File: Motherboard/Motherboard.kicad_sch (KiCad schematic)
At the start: 57 parts, among them J1 40-pin IDE Connector, J3 Bus_ISA_8bit, J4 ATX-24, J5 USB_B, J6 ATF15XX_JTAG_ISP, J7 Bus_ISA_8bit, J8 65SIB_Connector, SW1 SW_Push, SW2 SW_SPST, U1 AS6C8008, U10 ATF1508AS-PLCC84, U11 74HCT245, U12 74HCT573, U13 8255, U14 WD65C22, U15 AS6C8008, U16 MCP2200-I-SO, U17 74HCT163, U18 LM7905_TO220, U19 GAL16V8, U2 74HCT04, U4 SST39SF040, U5 SST39SF040, U6 SST39SF040, U7 SST39SF040, U8 WD65C816S, U9 DS1813, X1 ACO-xxxMHz, X2 ACO-24MHz, X3 ACO-14.31818MHz

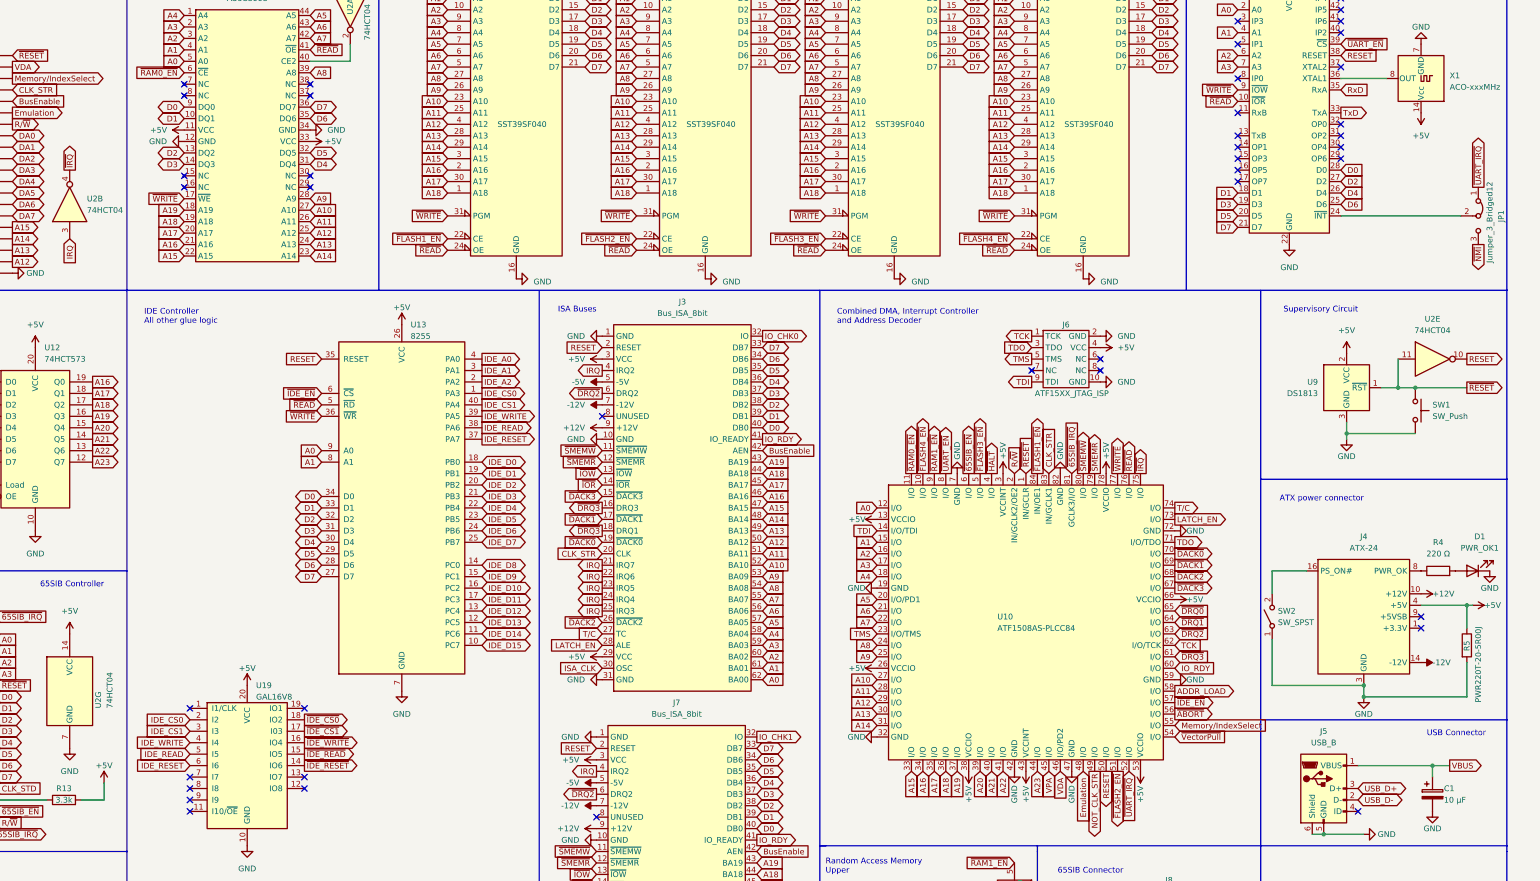
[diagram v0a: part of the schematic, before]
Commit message: Updated component footprints...
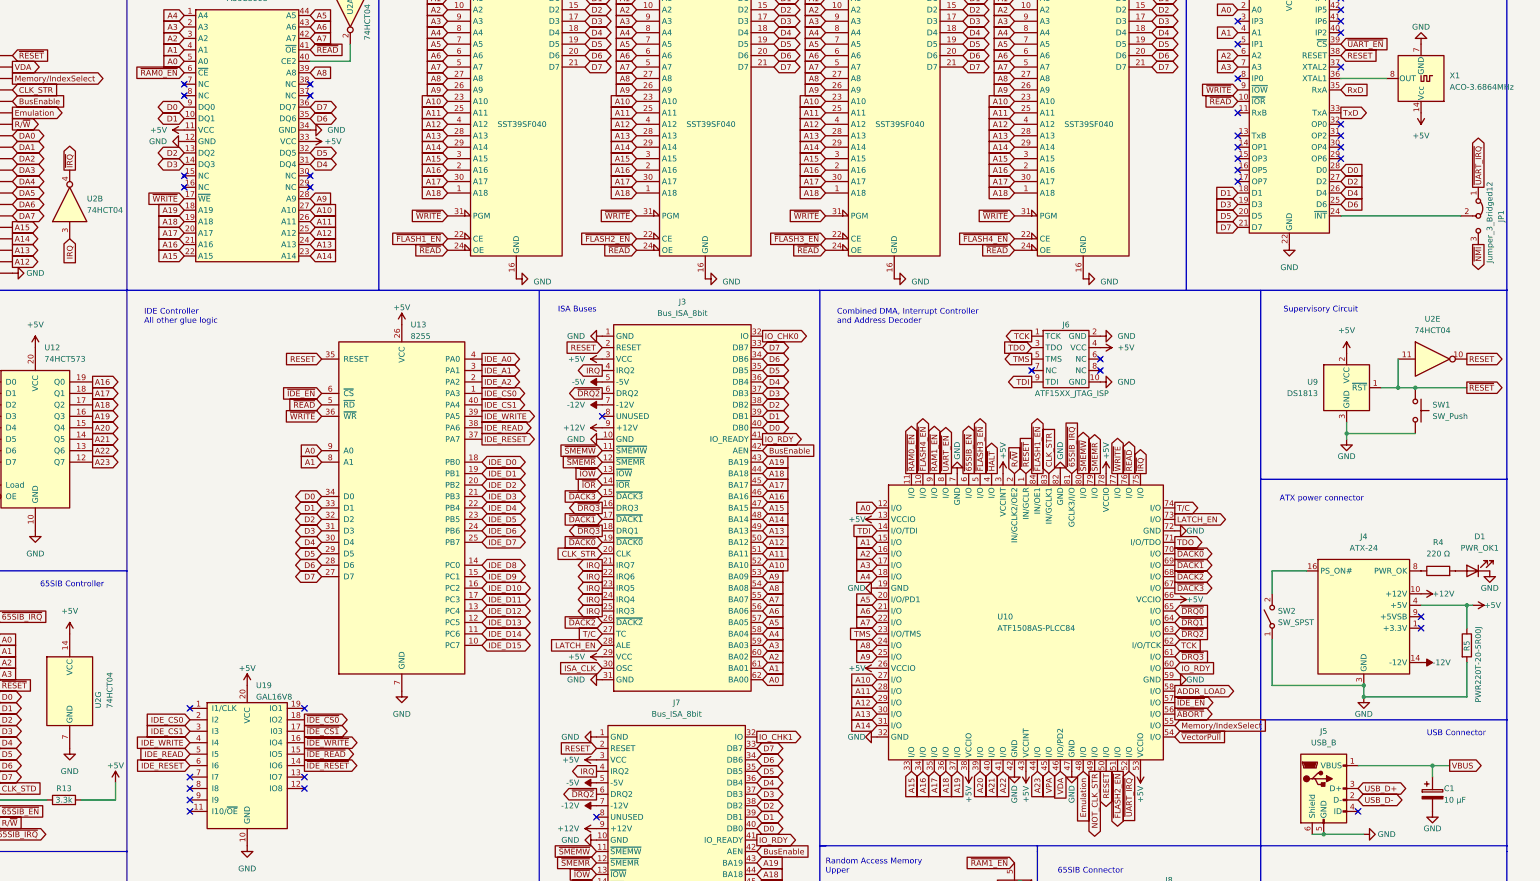
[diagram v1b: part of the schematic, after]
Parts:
- D7: footprint (none) -> LED_THT:LED_D5.0mm
- R12: footprint (none) -> Resistor_THT:R_Axial_DIN0207_L6.3mm_D2.5mm_P7.62mm_Horizontal
- U3: footprint (none) -> Package_LCC:PLCC-44_THT-Socket
- X1: value ACO-xxxMHz -> ACO-3.6864MHz
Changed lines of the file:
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@@
     (stroke (width 0) (type default))
   )
-  (wire (pts (xy 199.39 254) (xy 199.39 257.81))
+  (wire (pts (xy 201.93 254) (xy 201.93 257.81))
     (stroke (width 0) (type default))
   )
@@
     (stroke (width 0) (type default))
   )
-  (wire (pts (xy 194.31 257.81) (xy 199.39 257.81))
-    (stroke (width 0) (type default))
-  )
   (polyline (pts (xy 115.57 269.24) (xy 115.57 144.78))
     (stroke (width 0) (type default))
@@
     (stroke (width 0) (type default))
   )
+  (wire (pts (xy 194.31 257.81) (xy 201.93 257.81))
+    (stroke (width 0) (type default))
+  )
   (polyline (pts (xy 295.91 339.09) (xy 295.91 342.9))
     (stroke (width 0) (type default))
@@
       (effects (font (size 1.27 1.27)))
     )
-    (property "Footprint" "" (at 486.41 337.058 90)
+    (property "Footprint" "Resistor_THT:R_Axial_DIN0207_L6.3mm_D2.5mm_P7.62mm_Horizontal" (at 486.41 337.058 90)
       (effects (font (size 1.27 1.27)) hide)
     )
@@
       (effects (font (size 1.27 1.27)) (justify right))
     )
-    (property "Value" "ACO-xxxMHz" (at 497.84 99.695 0)
+    (property "Value" "ACO-3.6864MHz" (at 497.84 99.695 0)
       (effects (font (size 1.27 1.27)) (justify right))
     )
@@
       (effects (font (size 1.27 1.27)))
     )
-    (property "Footprint" "" (at 462.28 76.2 0)
+    (property "Footprint" "Package_LCC:PLCC-44_THT-Socket" (at 462.28 76.2 0)
       (effects (font (size 1.27 1.27)) hide)
     )
@@
     )
   )
-  (symbol (lib_name "+5V_5") (lib_id "power:+5V") (at 199.39 254 0) (unit 1)
+  (symbol (lib_name "+5V_5") (lib_id "power:+5V") (at 201.93 254 0) (unit 1)
     (in_bom yes) (on_board yes) (dnp no) (fields_autoplaced)
-    (property "Reference" "#PWR052" (at 199.39 257.81 0)
+    (property "Reference" "#PWR052" (at 201.93 257.81 0)
       (effects (font (size 1.27 1.27)) hide)
     )
-    (property "Value" "+5V" (at 199.39 250.19 0)
+    (property "Value" "+5V" (at 201.93 250.19 0)
       (effects (font (size 1.27 1.27)))
     )
-    (property "Footprint" "" (at 199.39 254 0)
+    (property "Footprint" "" (at 201.93 254 0)
       (effects (font (size 1.27 1.27)) hide)
     )
-    (property "Datasheet" "" (at 199.39 254 0)
+    (property "Datasheet" "" (at 201.93 254 0)
       (effects (font (size 1.27 1.27)) hide)
     )
@@
       (effects (font (size 1.27 1.27)))
     )
-    (property "Footprint" "" (at 494.03 335.28 0)
+    (property "Footprint" "LED_THT:LED_D5.0mm" (at 494.03 335.28 0)
       (effects (font (size 1.27 1.27)) hide)
     )

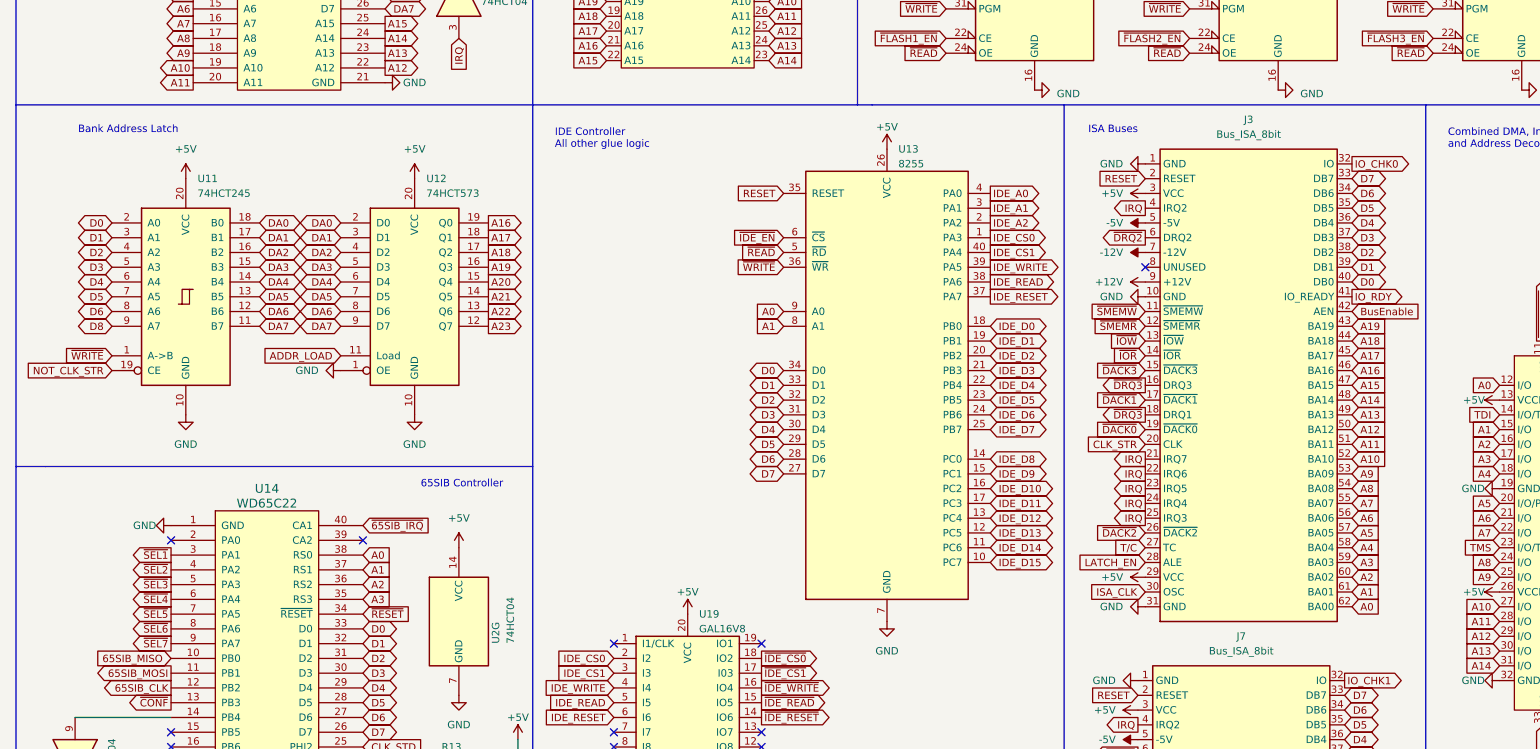
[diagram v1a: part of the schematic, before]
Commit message: Fixed D7 line...
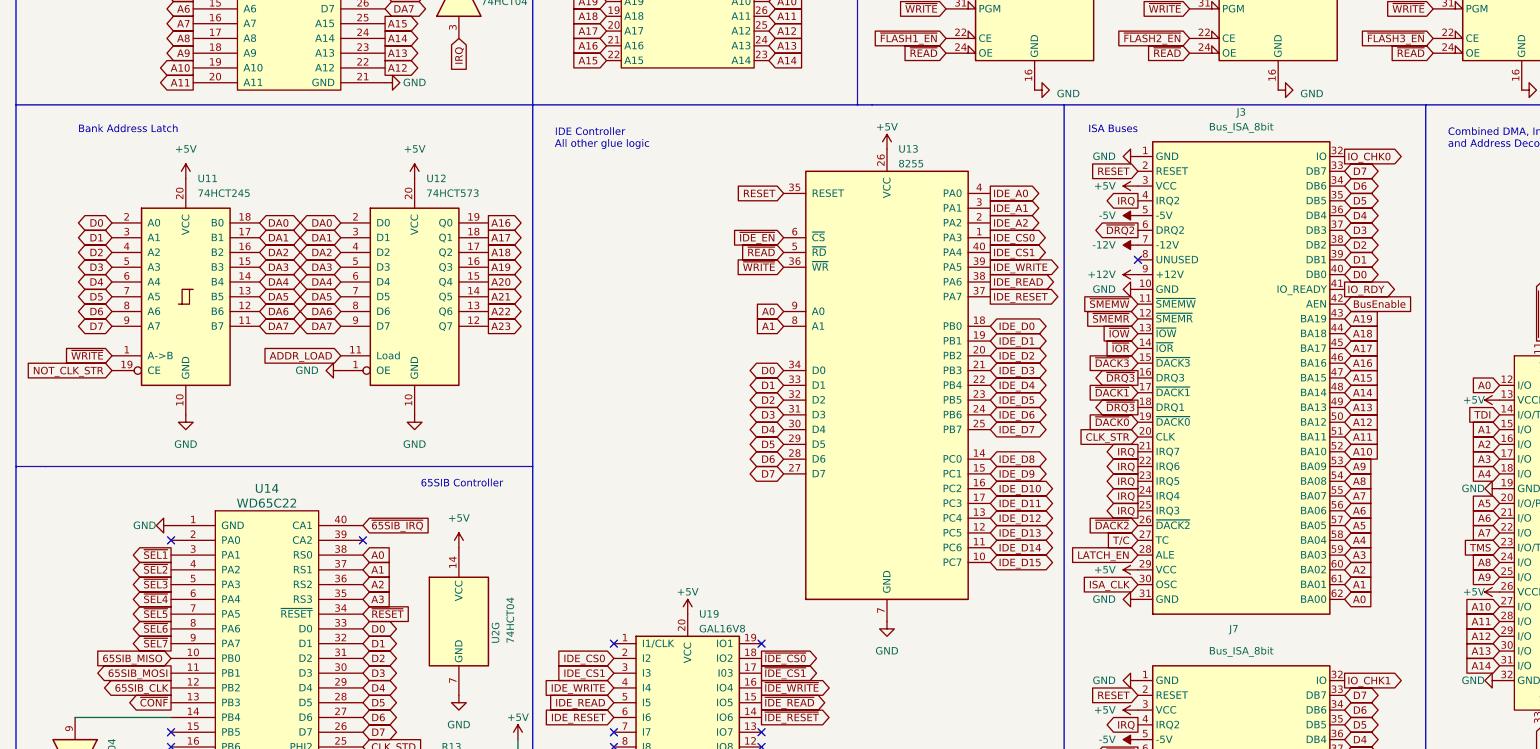
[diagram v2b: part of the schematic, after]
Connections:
- net D8 is gone; now on net D7: U11.9 (A7)
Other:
- moved on the sheet: J3
